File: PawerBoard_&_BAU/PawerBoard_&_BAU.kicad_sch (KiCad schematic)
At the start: 83 parts, among them IC1 MC34167TG, J1 Conn_01x02, J10 Conn_01x02, J11 Conn_01x02, J12 Conn_01x02, J2 XT60-M, J3 Conn_01x02, J4 Conn_01x02, J5 Conn_01x02, J6 Conn_01x02, J7 Conn_01x02, J8 Screw_Terminal_01x08, J9 Conn_01x02, K1 TE_PCH-1xxx2M, Q1 IRLIZ44N, Q2 IRLIZ44N, U1 L78L05_TO92, U10 LM2596-Dsun, U11 LM2576T-5, U12 LM2596-Dsun, U2 NE555P, U4 74LS04, U5 L78L12_TO92, U7 Gege_buzer, U8 LM2596-Dsun

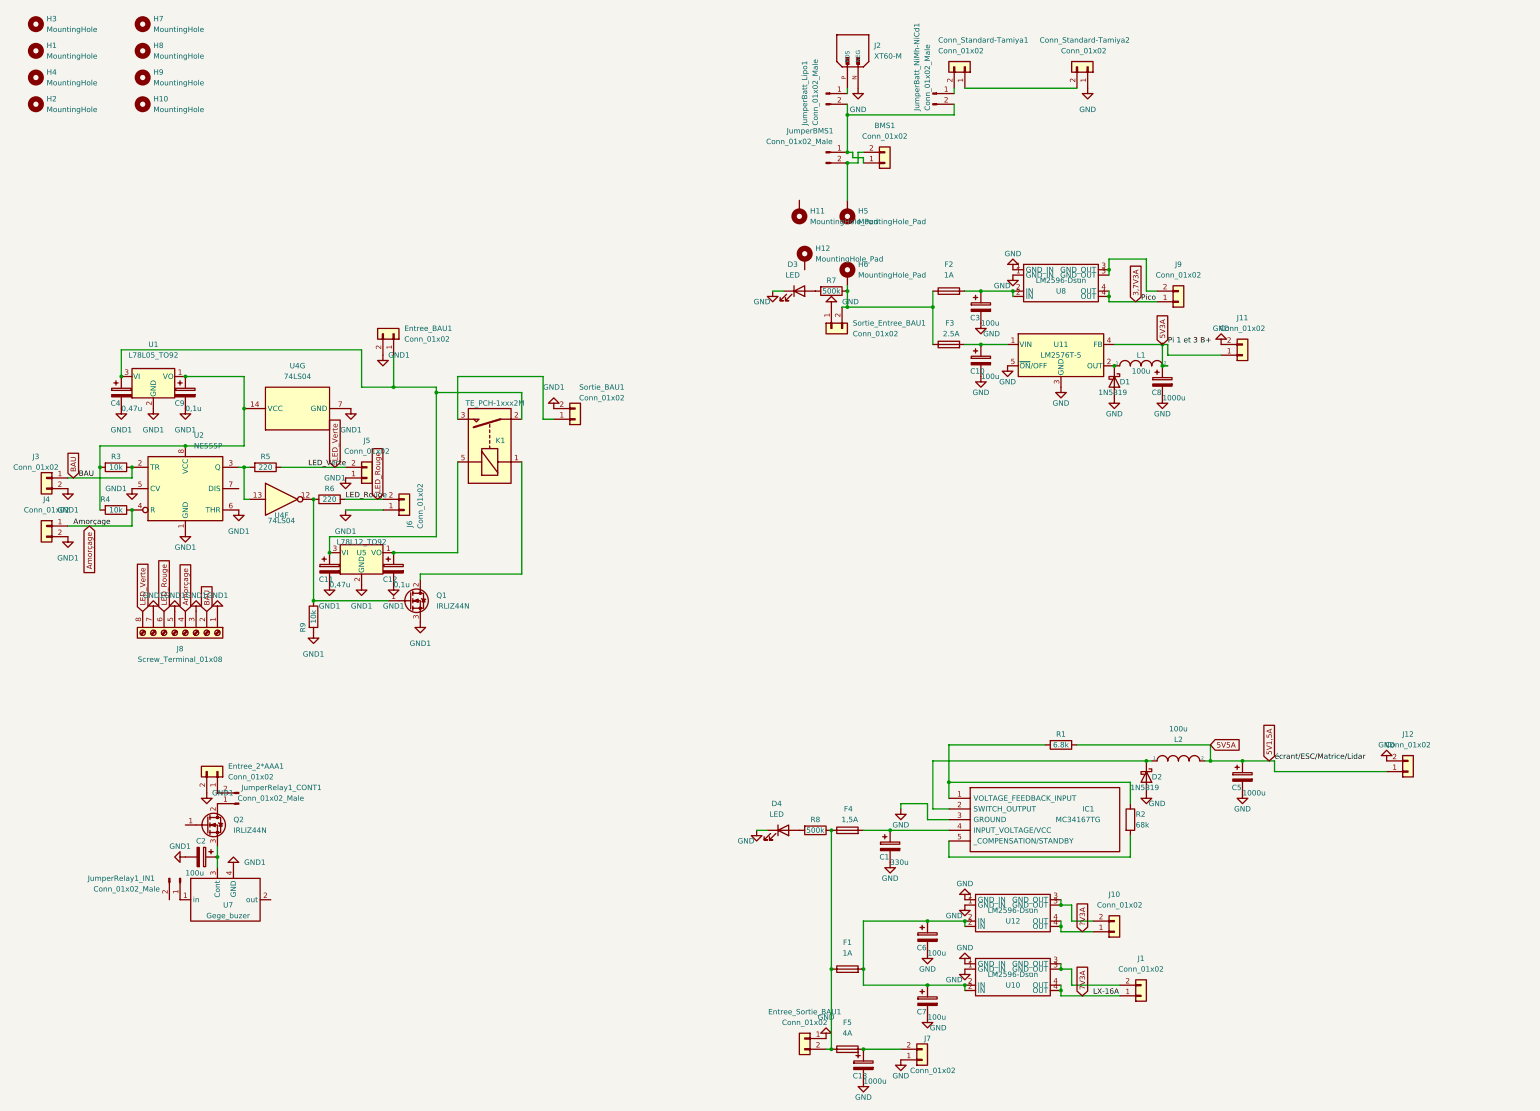
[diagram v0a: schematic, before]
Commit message: Feat: add assets
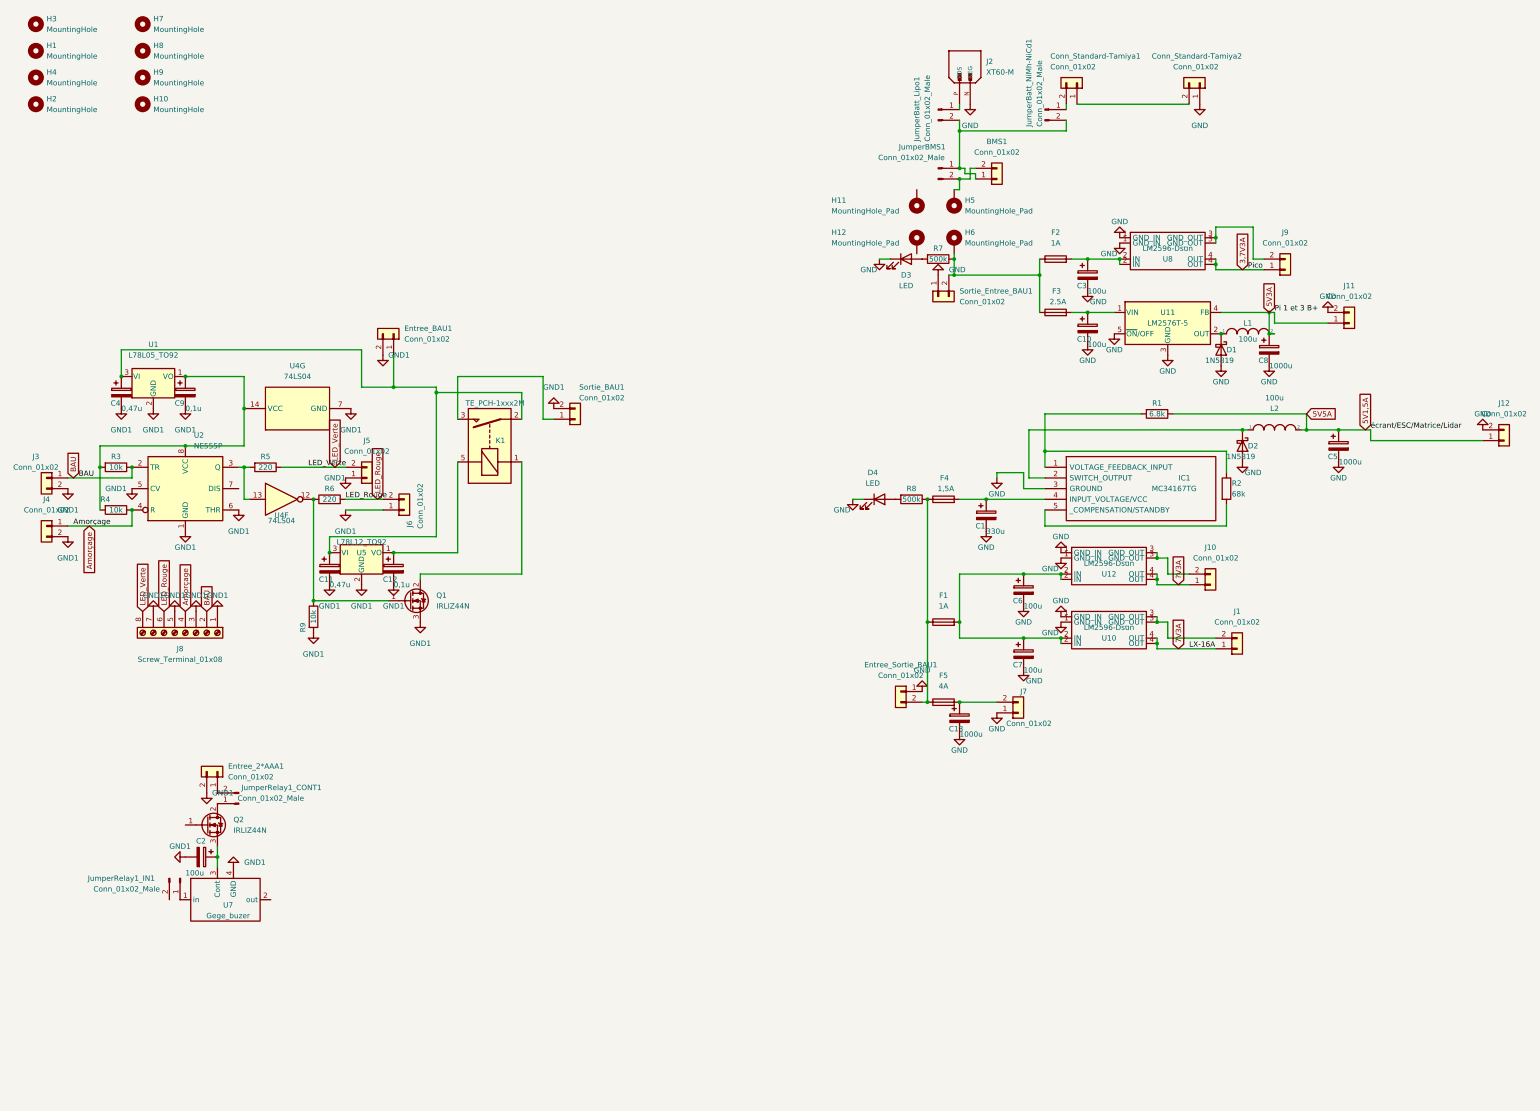
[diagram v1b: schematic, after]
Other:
- moved on the sheet: BMS1, C1, C10, C13, C3, C5, C6, C7, C8, Conn_Standard-Tamiya1, Conn_Standard-Tamiya2, D1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
